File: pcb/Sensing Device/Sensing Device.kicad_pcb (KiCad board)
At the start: 2 copper layers, 100 x 60 mm, 20 parts, among them J1 PWR_PAD, J2 ID_PAD, SW1 SW_SPST, SW2 SW_SPDT, U2 TLV493D

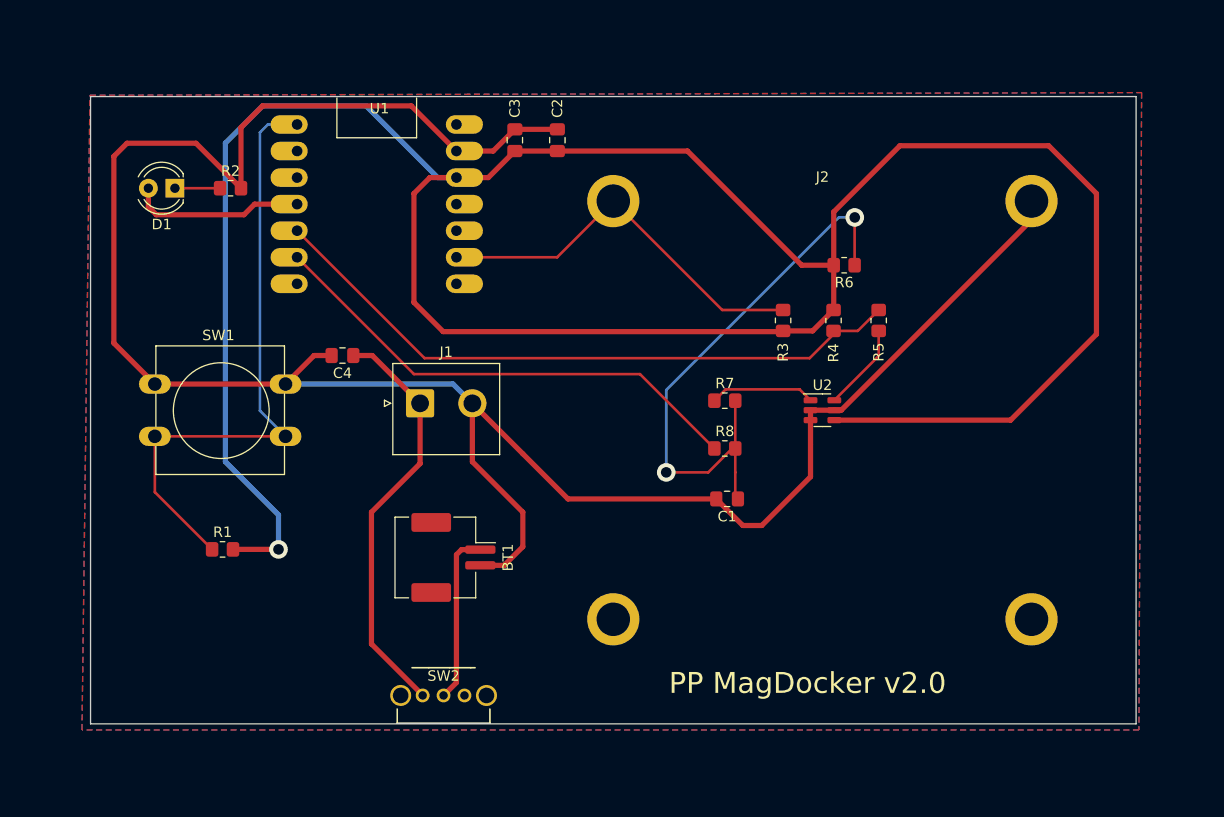
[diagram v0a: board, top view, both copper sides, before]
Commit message: readme
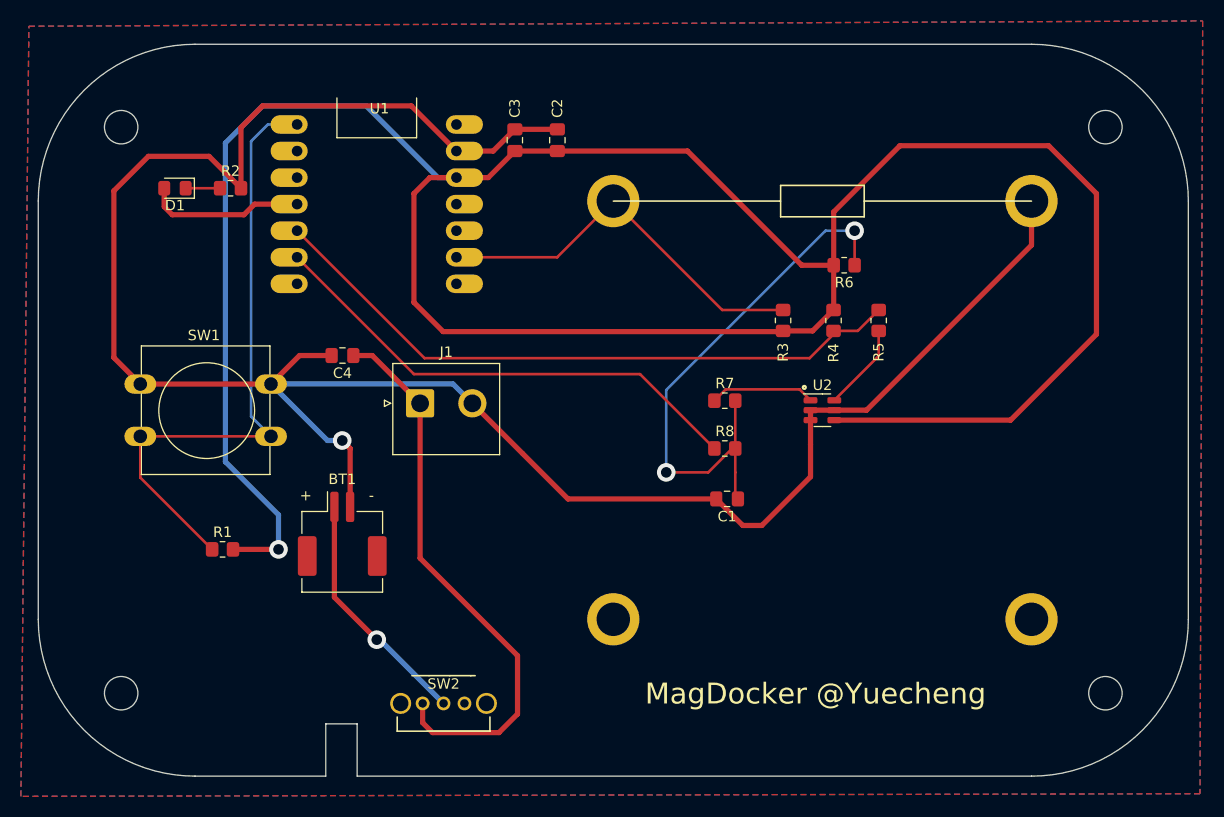
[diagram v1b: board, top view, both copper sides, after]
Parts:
- D1: value LED -> LS R976; footprint LED_THT:LED_D4.0mm -> LED_SMD:LED_0805_2012Metric_Pad1.15x1.40mm_HandSolder
- R2: value 50Ω -> 65Ω
- moved BT1 10.9 mm to (84.1, 81.8), turned to 0 degrees
- moved SW1 1.39 mm to (64.8, 67.5)
- moved SW2 0.76 mm to (91.8, 98.0)
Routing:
- net VCC: track 40.2 -> 54.3 mm
- net Net-(BT1-+): track 16.5 -> 23.3 mm, vias 0 -> 1
- net GND: track 210.6 -> 205.0 mm, vias 0 -> 1
- net Net-(C1-Pad1): track 53.8 -> 52.0 mm
- net /LED: track 16.7 -> 15.2 mm
- net Net-(D1-K): track 4.32 -> 3.29 mm
- net /Button: track 60.6 -> 61.3 mm
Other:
- board size 100 x 60 mm -> 110 x 70 mm
- board text added: "+"
- board text added: "-"
- board text added: "MagDocker @Yuecheng"
- board text removed: "PP MagDocker v2.0"
